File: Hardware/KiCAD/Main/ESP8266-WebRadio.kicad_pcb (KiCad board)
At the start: 2 copper layers, 52.5 x 36.6 mm, 52 parts, among them K1 AUDIO, K2 POWER, K3 EARPHONES, P1 UART, P2 PROG, U1 LM1117-3.3, U2 LM1117-1.8, U3 23LCV1024, U4 ESP8266_ESP-12, U5 NE5532, U6 VS1053, X1 12.288MHz

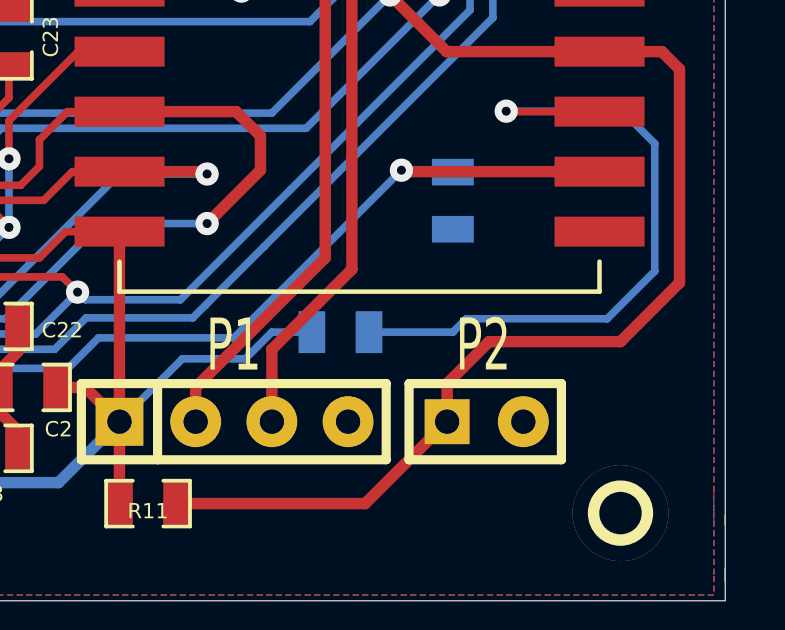
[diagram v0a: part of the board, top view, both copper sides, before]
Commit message: Monitor is now better
A little memory leaks.
Updated hardware from piotr.
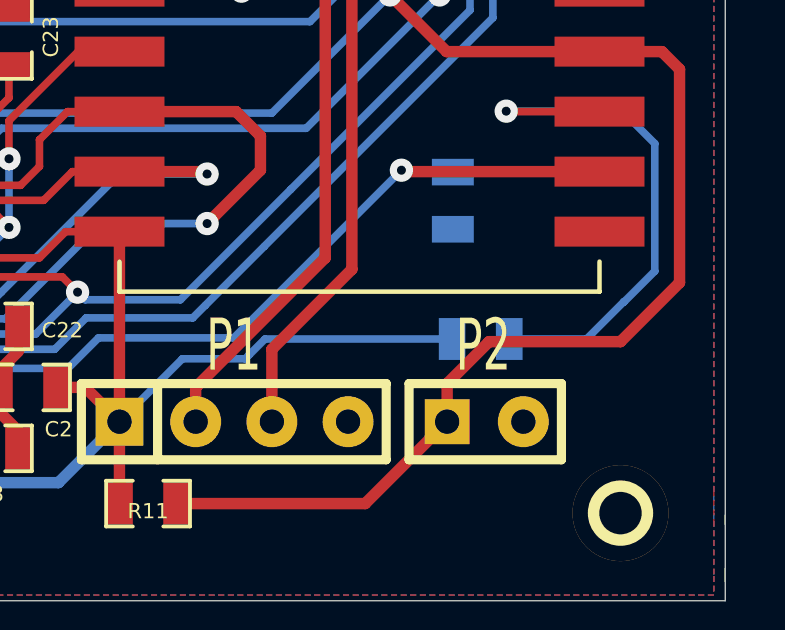
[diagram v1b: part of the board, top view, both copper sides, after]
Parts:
- moved R12 4.68 mm to (58.9, 42.8)
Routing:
- net +3.3V: track 140.7 -> 145.3 mm
- net N-0000017: track 23.1 -> 18.6 mm
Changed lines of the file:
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@@
     (links 139)
     (no_connects 0)
-    (area 14.599999 14.980999 67.061001 51.567001)
+    (area 14.599999 14.7828 67.061001 51.71694)
     (thickness 1.6)
     (drawings 10)
-    (tracks 484)
+    (tracks 485)
     (zones 0)
     (modules 52)
@@
     (18 B.Paste user)
     (19 F.Paste user)
-    (20 B.SilkS user hide)
+    (20 B.SilkS user)
     (21 F.SilkS user)
     (22 B.Mask user)
@@
   )
   (module SM0805 (layer B.Cu)
-    (at 54.229 42.6085)
+    (at 58.9026 42.8371)
     (attr smd)
     (fp_text reference R12 (at 0 0.254) (layer B.SilkS)
@@
   (segment (start 33.655 37.211) (end 33.655 37.592) (width 0.254) (layer F.Cu) (net 1))
   (segment (start 33.53308 37.71392) (end 32.60598 37.71392) (width 0.254) (layer F.Cu) (net 1))
-  (segment (start 53.2765 42.6085) (end 51.943 42.6085) (width 0.254) (layer B.Cu) (net 2))
+  (segment (start 57.9501 42.8371) (end 51.7144 42.8371) (width 0.254) (layer B.Cu) (net 2))
+  (segment (start 51.7144 42.8371) (end 51.181 43.3705) (width 0.254) (layer B.Cu) (net 2))
   (segment (start 48.9585 43.4975) (end 46.863 45.593) (width 0.254) (layer B.Cu) (net 2))
   (segment (start 51.054 43.4975) (end 48.9585 43.4975) (width 0.254) (layer B.Cu) (net 2))
-  (segment (start 51.943 42.6085) (end 51.054 43.4975) (width 0.254) (layer B.Cu) (net 2))
+  (segment (start 51.181 43.3705) (end 51.054 43.4975) (width 0.254) (layer B.Cu) (net 2))
   (segment (start 46.863 48.3235) (end 46.863 45.593) (width 0.381) (layer F.Cu) (net 2))
   (segment (start 30.734 38.989) (end 30.988 38.735) (width 0.254) (layer F.Cu) (net 2))
@@
   (segment (start 18.923 19.05) (end 18.923 17.653) (width 0.381) (layer F.Cu) (net 11))
   (segment (start 18.923 17.653) (end 19.558 17.018) (width 0.381) (layer F.Cu) (net 11))
-  (segment (start 55.1815 42.6085) (end 57.9755 42.6085) (width 0.254) (layer B.Cu) (net 12))
+  (segment (start 59.8551 42.8371) (end 62.4332 42.8371) (width 0.254) (layer B.Cu) (net 12))
+  (segment (start 63.6778 41.5925) (end 63.6778 41.6052) (width 0.254) (layer B.Cu) (net 12))
+  (segment (start 62.4332 42.8371) (end 63.6778 41.5925) (width 0.254) (layer B.Cu) (net 12))
   (segment (start 59.769 35.258) (end 62.864 35.258) (width 0.254) (layer F.Cu) (net 12))
   (segment (start 59.7535 35.2425) (end 59.769 35.258) (width 0.254) (layer F.Cu) (net 12))
@@
   (segment (start 64.7065 36.322) (end 63.627 35.2425) (width 0.254) (layer B.Cu) (net 12))
   (segment (start 64.7065 40.5765) (end 64.7065 36.322) (width 0.254) (layer B.Cu) (net 12))
-  (segment (start 63.119 42.164) (end 64.7065 40.5765) (width 0.254) (layer B.Cu) (net 12))
-  (segment (start 58.42 42.164) (end 63.119 42.164) (width 0.254) (layer B.Cu) (net 12))
-  (segment (start 57.9755 42.6085) (end 58.42 42.164) (width 0.254) (layer B.Cu) (net 12))
+  (segment (start 63.6778 41.6052) (end 64.7065 40.5765) (width 0.254) (layer B.Cu) (net 12))
   (segment (start 35.9537 41.56202) (end 35.9537 45.3898) (width 0.254) (layer F.Cu) (net 13))
   (segment (start 35.9537 45.3898) (end 35.7505 45.593) (width 0.254) (layer F.Cu) (net 13))
